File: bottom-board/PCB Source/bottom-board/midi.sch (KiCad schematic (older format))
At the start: 14 parts, among them P6 AudioJack3, P7 AudioJack3, Q12 2N7002, Q13 2N7002, U11 6N137S

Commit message: change design to 4 layer PCB
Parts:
- R47, R49, R50: MPN RL73N1JR22JTD -> RC0603FR-07220RL
- U11: footprint Package_DIP:DIP-8_W7.62mm_SMDSocket_SmallPads -> Uno:6N137S
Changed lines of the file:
@@
 F 2 "Resistor_SMD:R_0603_1608Metric" H 6665 3335 60  0001 C CNN
 F 3 "" H 6665 3335 60  0000 C CNN
-F 4 "RL73N1JR22JTD" H 365 -15 50  0001 C CNN "MPN"
+F 4 "RC0603FR-07220RL" H 365 -15 50  0001 C CNN "MPN"
 	1    6665 3335
 	0    1    1    0
@@
 F 2 "Resistor_SMD:R_0603_1608Metric" H 7700 3550 60  0001 C CNN
 F 3 "" H 7700 3550 60  0000 C CNN
-F 4 "RL73N1JR22JTD" H 350 0   50  0001 C CNN "MPN"
+F 4 "RC0603FR-07220RL" H 350 0   50  0001 C CNN "MPN"
 	1    7700 3550
 	0    -1   -1   0
@@
 F 0 "U11" H 3570 3520 50  0000 L CNN
 F 1 "6N137S" H 3820 3520 50  0000 L CNN
-F 2 "Package_DIP:DIP-8_W7.62mm_SMDSocket_SmallPads" H 3620 3520 50  0001 L CIN
+F 2 "Uno:6N137S" H 3620 3520 50  0001 L CIN
 F 3 "" H 3820 3820 50  0000 L CNN
 F 4 "6N137S" H 170 170 50  0001 C CNN "MPN"
@@
 F 2 "Resistor_SMD:R_0603_1608Metric" H 2920 3720 60  0001 C CNN
 F 3 "" H 2920 3720 60  0000 C CNN
-F 4 "RL73N1JR22JTD" H -3380 370 50  0001 C CNN "MPN"
+F 4 "RC0603FR-07220RL" H -3380 370 50  0001 C CNN "MPN"
 	1    2920 3720
 	0    -1   -1   0

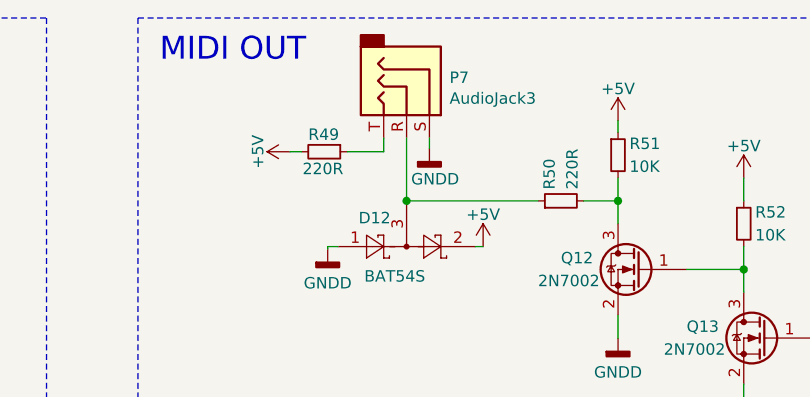
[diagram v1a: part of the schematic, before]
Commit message: minor cleanup
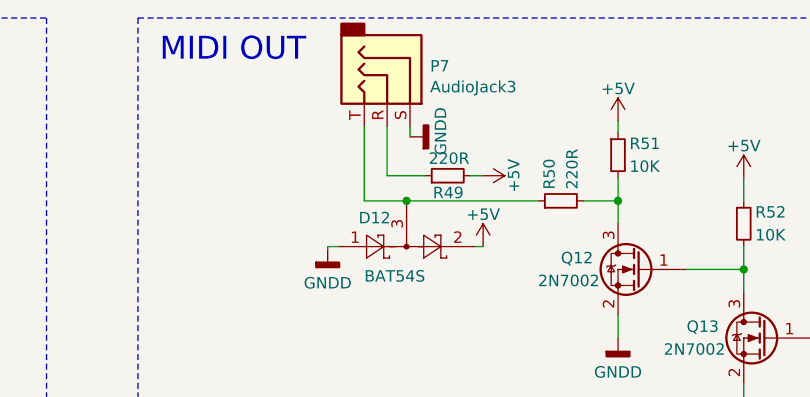
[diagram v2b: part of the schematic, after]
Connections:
- net at R49.1: now also P7.R; no longer P7.T
- net at D12.3, R50.1: now also P7.T; no longer P7.R
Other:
- moved on the sheet: P7, R49
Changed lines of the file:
@@
 L bottom-board-rescue:R_Small R49
 U 1 1 550EE5CB
-P 6665 3335
-F 0 "R49" V 6590 3265 50  0000 L CNN
-F 1 "220R" V 6740 3240 50  0000 L CNN
-F 2 "Resistor_SMD:R_0603_1608Metric" H 6665 3335 60  0001 C CNN
-F 3 "" H 6665 3335 60  0000 C CNN
-F 4 "RC0603FR-07220RL" H 365 -15 50  0001 C CNN "MPN"
-	1    6665 3335
-	0    1    1    0
+P 7205 3440
+F 0 "R49" V 7130 3370 50  0000 L CNN
+F 1 "220R" V 7280 3345 50  0000 L CNN
+F 2 "Resistor_SMD:R_0603_1608Metric" H 7205 3440 60  0001 C CNN
+F 3 "" H 7205 3440 60  0000 C CNN
+F 4 "RC0603FR-07220RL" H 905 90  50  0001 C CNN "MPN"
+	1    7205 3440
+	0    -1   -1   0
 $EndComp
 $Comp
@@
 L bottom-board-rescue:GNDD-power #PWR0185
 U 1 1 550D24C3
-P 7125 3320
-F 0 "#PWR0185" H 7125 3070 50  0001 C CNN
-F 1 "GNDD" H 7150 3185 50  0000 C CNN
-F 2 "" H 7125 3320 60  0000 C CNN
-F 3 "" H 7125 3320 60  0000 C CNN
-	1    7125 3320
-	1    0    0    -1
+P 7040 3270
+F 0 "#PWR0185" H 7040 3020 50  0001 C CNN
+F 1 "GNDD" H 7065 3135 50  0000 C CNN
+F 2 "" H 7040 3270 60  0000 C CNN
+F 3 "" H 7040 3270 60  0000 C CNN
+	1    7040 3270
+	0    -1   -1   0
 $EndComp
 $Comp
@@
 L bottom-board-rescue:+5V-power #PWR0189
 U 1 1 550D42BC
-P 6515 3335
-F 0 "#PWR0189" H 6515 3185 50  0001 C CNN
-F 1 "+5V" H 6515 3475 50  0000 C CNN
-F 2 "" H 6515 3335 60  0000 C CNN
-F 3 "" H 6515 3335 60  0000 C CNN
-	1    6515 3335
-	0    -1   -1   0
+P 7355 3440
+F 0 "#PWR0189" H 7355 3290 50  0001 C CNN
+F 1 "+5V" H 7355 3580 50  0000 C CNN
+F 2 "" H 7355 3440 60  0000 C CNN
+F 3 "" H 7355 3440 60  0000 C CNN
+	1    7355 3440
+	0    1    1    0
 $EndComp
 $Comp
@@
 	5850 2750 9950 2750
 Wire Wire Line
-	6565 3335 6515 3335
+	7305 3440 7355 3440
 Wire Wire Line
 	7950 3200 7950 3250
@@
 Wire Wire Line
 	8500 3850 8500 3950
-$Comp
-L bottom-board-rescue:AudioJack3-Connector P6
-U 1 1 5D15D509
-P 2345 3445
-F 0 "P6" V 2373 3215 50  0000 R CNN
-F 1 "AudioJack3" V 2045 3595 50  0000 R CNN
-F 2 "Connector_Audio:Jack_3.5mm_CUI_SJ-3523-SMT_Horizontal" H 2345 3445 50  0001 C CNN
-F 3 "~" H 2345 3445 50  0001 C CNN
-F 4 "SJ-3523-SMT-TR" V 2345 3445 50  0001 C CNN "MPN"
-	1    2345 3445
-	0    1    1    0
-$EndComp
-NoConn ~ 2445 3645
 $Comp
 L bottom-board-rescue:1N4148-Diode D?
@@
 $EndComp
 Wire Wire Line
-	2820 3720 2345 3720
-Wire Wire Line
-	2345 3720 2345 3645
-Wire Wire Line
-	3320 4205 3220 4205
-Wire Wire Line
-	2245 4205 2245 3645
-Wire Wire Line
-	3320 3920 3320 4205
-Wire Wire Line
-	3220 4070 3220 4205
-Connection ~ 3220 4205
-Wire Wire Line
-	3220 4205 2245 4205
-Wire Wire Line
 	4120 3620 4230 3620
 Wire Wire Line
@@
 L bottom-board-rescue:AudioJack3-Connector P7
 U 1 1 5D15C2EF
-P 7025 3075
-F 0 "P7" V 6961 3263 50  0000 L CNN
-F 1 "AudioJack3" V 7052 3263 50  0000 L CNN
-F 2 "Connector_Audio:Jack_3.5mm_CUI_SJ-3523-SMT_Horizontal" H 7025 3075 50  0001 C CNN
-F 3 "~" H 7025 3075 50  0001 C CNN
-F 4 "SJ-3523-SMT-TR" V 7025 3075 50  0001 C CNN "MPN"
-	1    7025 3075
+P 6940 3025
+F 0 "P7" V 6876 3213 50  0000 L CNN
+F 1 "AudioJack3" V 6967 3213 50  0000 L CNN
+F 2 "Connector_Audio:Jack_3.5mm_CUI_SJ-3523-SMT_Horizontal" H 6940 3025 50  0001 C CNN
+F 3 "~" H 6940 3025 50  0001 C CNN
+F 4 "SJ-3523-SMT-TR" V 6940 3025 50  0001 C CNN "MPN"
+	1    6940 3025
 	0    1    1    0
 $EndComp
@@
 	7600 3550 7025 3550
 Wire Wire Line
-	7025 3550 7025 3275
-Wire Wire Line
-	7125 3320 7125 3275
-Wire Wire Line
-	6925 3335 6925 3275
-Wire Wire Line
-	6765 3335 6925 3335
+	7040 3270 7040 3225
 Wire Notes Line
 	5450 4695 1600 4695
@@
 	1    0    0    1
 $EndComp
-Connection ~ 7025 3550
 $Comp
 L bottom-board-rescue:+5V-power #PWR0265
@@
 Wire Wire Line
 	7325 3750 7360 3750
+Wire Wire Line
+	3320 3920 3320 4205
+Wire Wire Line
+	3320 4205 3220 4205
+Wire Wire Line
+	3220 4070 3220 4205
+NoConn ~ 2445 3645
+$Comp
+L bottom-board-rescue:AudioJack3-Connector P6
+U 1 1 5D15D509
+P 2345 3445
+F 0 "P6" V 2373 3215 50  0000 R CNN
+F 1 "AudioJack3" V 2045 3595 50  0000 R CNN
+F 2 "Connector_Audio:Jack_3.5mm_CUI_SJ-3523-SMT_Horizontal" H 2345 3445 50  0001 C CNN
+F 3 "~" H 2345 3445 50  0001 C CNN
+F 4 "SJ-3523-SMT-TR" V 2345 3445 50  0001 C CNN "MPN"
+	1    2345 3445
+	0    1    1    0
+$EndComp
+Connection ~ 3220 4205
+Wire Wire Line
+	3220 4205 2245 4205
+Wire Wire Line
+	2245 4205 2245 3645
+Wire Wire Line
+	2345 3720 2345 3645
+Wire Wire Line
+	2820 3720 2345 3720
+Wire Wire Line
+	6940 3225 6940 3440
+Wire Wire Line
+	6940 3440 7105 3440
+Wire Wire Line
+	6840 3225 6840 3550
+Wire Wire Line
+	6840 3550 7025 3550
+Connection ~ 7025 3550
 $EndSCHEMATC
